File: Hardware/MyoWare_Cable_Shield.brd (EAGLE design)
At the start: 52.3 x 20.8 mm, 16 parts

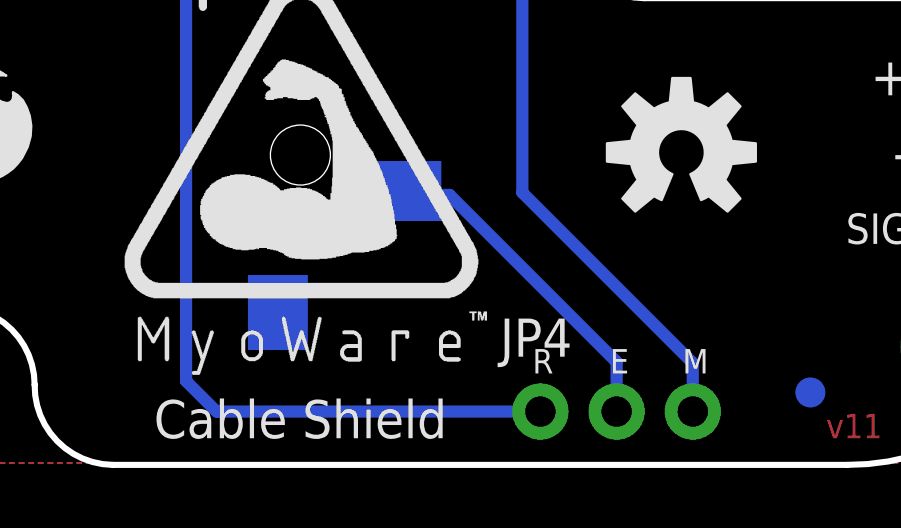
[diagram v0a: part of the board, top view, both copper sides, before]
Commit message: Minor Adjustment
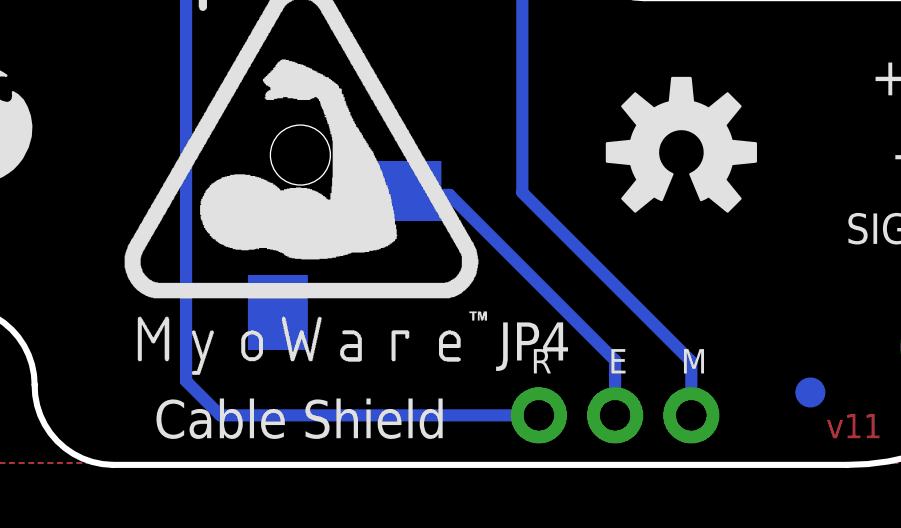
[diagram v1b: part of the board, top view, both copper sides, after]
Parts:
- moved JP4 0.14 mm to (34.1, 1.65)
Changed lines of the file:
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@@
 <?xml version="1.0" encoding="utf-8"?>
 <!DOCTYPE eagle SYSTEM "eagle.dtd">
-<eagle version="7.2.0">
+<eagle version="7.7.0">
 <drawing>
 <settings>
@@
 <wire x1="19.90725" y1="0" x2="44.3865" y2="0" width="0.2032" layer="20"/>
 <wire x1="32.41675" y1="20.828" x2="7.9375" y2="20.828" width="0.2032" layer="20"/>
-<text x="39.3319" y="3.048" size="0.8128" layer="21" font="vector" ratio="20" align="bottom-center">M</text>
-<text x="34.24555" y="3.048" size="0.8128" layer="21" font="vector" ratio="20" align="bottom-center">R</text>
-<text x="36.79825" y="3.048" size="0.8128" layer="21" font="vector" ratio="20" align="bottom-center">E</text>
+<text x="39.2811" y="3.048" size="0.8128" layer="21" font="vector" ratio="20" align="bottom-center">M</text>
+<text x="34.19475" y="3.048" size="0.8128" layer="21" font="vector" ratio="20" align="bottom-center">R</text>
+<text x="36.74745" y="3.048" size="0.8128" layer="21" font="vector" ratio="20" align="bottom-center">E</text>
 <text x="6.4262" y="12.954" size="1.016" layer="21" font="vector" ratio="17" align="center-left">RAW</text>
 <text x="6.4262" y="10.414" size="1.016" layer="21" font="vector" ratio="17" align="center-left">SHLD</text>
@@
 <text x="6.2738" y="10.414" size="1.016" layer="22" font="vector" ratio="17" rot="MR0" align="center-right">SHLD</text>
 <text x="6.2738" y="7.874" size="1.016" layer="22" font="vector" ratio="17" rot="MR0" align="center-right">GND</text>
-<text x="39.17315" y="3.048" size="0.8128" layer="22" font="vector" ratio="20" rot="MR0" align="bottom-center">M</text>
-<text x="34.09315" y="3.048" size="0.8128" layer="22" font="vector" ratio="20" rot="MR0" align="bottom-center">R</text>
-<text x="36.63315" y="3.048" size="0.8128" layer="22" font="vector" ratio="20" rot="MR0" align="bottom-center">E</text>
+<text x="39.12235" y="3.048" size="0.8128" layer="22" font="vector" ratio="20" rot="MR0" align="bottom-center">M</text>
+<text x="34.04235" y="3.048" size="0.8128" layer="22" font="vector" ratio="20" rot="MR0" align="bottom-center">R</text>
+<text x="36.58235" y="3.048" size="0.8128" layer="22" font="vector" ratio="20" rot="MR0" align="bottom-center">E</text>
 <wire x1="50.673" y1="15.5575" x2="52.324" y2="14.0335" width="0.2032" layer="20" curve="-90"/>
 <dimension x1="-6.25475" y1="-10.414" x2="-18.2245" y2="10.414" x3="-34.29" y3="0" textsize="1.778" textratio="15" layer="47" dtype="vertical" unit="inch"/>
@@
 <element name="LOGO" library="advancer-technologies" package="MYOWARE_LOGO" value="" x="26.162" y="9.525"/>
 <element name="SPIRAL" library="advancer-technologies" package="SPIRAL_LOGO_60%" value="" x="22.9489" y="17.7927"/>
-<element name="JP4" library="SparkFun-Connectors" package="1X03_NO_SILK" value="Power" x="34.163" y="1.778"/>
+<element name="JP4" library="SparkFun-Connectors" package="1X03_NO_SILK" value="Power" x="34.1122" y="1.651"/>
 <element name="JP5" library="SparkFun-Connectors" package="1X03_NO_SILK" value="Power" x="50.7365" y="12.954" rot="R270"/>
 <element name="JP2" library="SparkFun-Connectors" package="1X03_NO_SILK" value="Power" x="1.5875" y="12.954" rot="R270"/>
@@
 <contactref element="JP4" pad="3"/>
 <wire x1="33.55975" y1="16.98625" x2="33.55975" y2="9.077959375" width="0.4064" layer="16"/>
-<wire x1="33.55975" y1="9.077959375" x2="39.243" y2="3.394709375" width="0.4064" layer="16"/>
+<wire x1="33.55975" y1="9.077959375" x2="39.1922" y2="3.445509375" width="0.4064" layer="16"/>
 <contactref element="JP3" pad="SLEEVE"/>
 <wire x1="29.612" y1="18.428" x2="32.118" y2="18.428" width="0.4064" layer="16"/>
 <wire x1="32.118" y1="18.428" x2="33.55975" y2="16.98625" width="0.4064" layer="16"/>
-<wire x1="39.243" y1="1.778" x2="39.243" y2="3.394709375" width="0.4064" layer="16"/>
+<wire x1="39.1922" y1="1.651" x2="39.1922" y2="3.445509375" width="0.4064" layer="16"/>
 </signal>
 <signal name="END">
 <contactref element="JP4" pad="2"/>
-<wire x1="36.703" y1="3.429" x2="31.133034375" y2="8.999" width="0.4064" layer="16"/>
+<wire x1="36.6522" y1="3.4798" x2="31.133034375" y2="8.999" width="0.4064" layer="16"/>
 <contactref element="JP3" pad="TIP"/>
 <wire x1="31.133034375" y1="8.999" x2="29.61513125" y2="8.999" width="0.4064" layer="16"/>
 <wire x1="29.61513125" y1="8.999" x2="29.612" y2="9.128" width="0.4064" layer="16"/>
-<wire x1="36.703" y1="1.778" x2="36.703" y2="3.429" width="0.4064" layer="16"/>
+<wire x1="36.6522" y1="1.651" x2="36.6522" y2="3.4798" width="0.4064" layer="16"/>
 </signal>
 <signal name="VREF">
 <contactref element="JP4" pad="1"/>
-<wire x1="34.163" y1="1.778" x2="23.368" y2="1.778" width="0.4064" layer="16"/>
-<wire x1="23.368" y1="1.778" x2="22.352" y2="2.794" width="0.4064" layer="16"/>
+<wire x1="34.1122" y1="1.651" x2="23.495" y2="1.651" width="0.4064" layer="16"/>
+<wire x1="23.495" y1="1.651" x2="22.352" y2="2.794" width="0.4064" layer="16"/>
 <wire x1="22.352" y1="2.794" x2="22.352" y2="16.389" width="0.4064" layer="16"/>
 <contactref element="JP3" pad="RING"/>

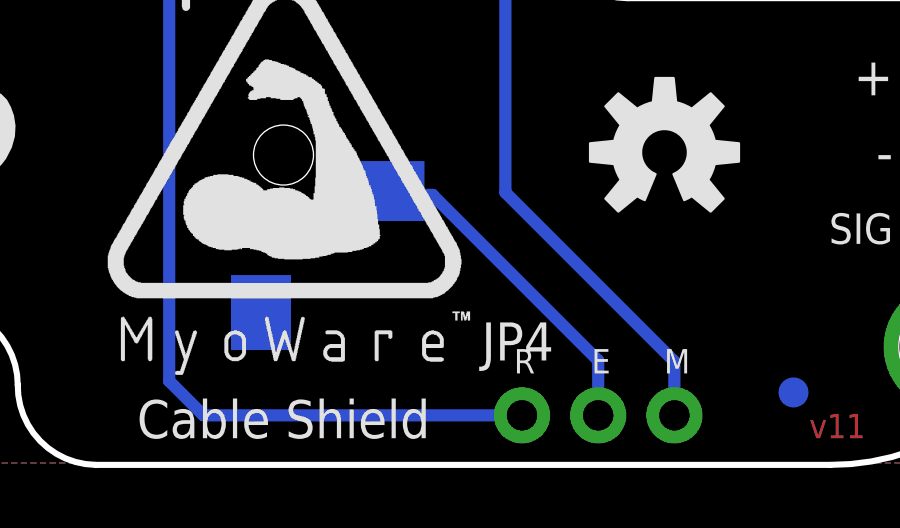
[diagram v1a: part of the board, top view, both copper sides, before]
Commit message: Final Adjust before Protos
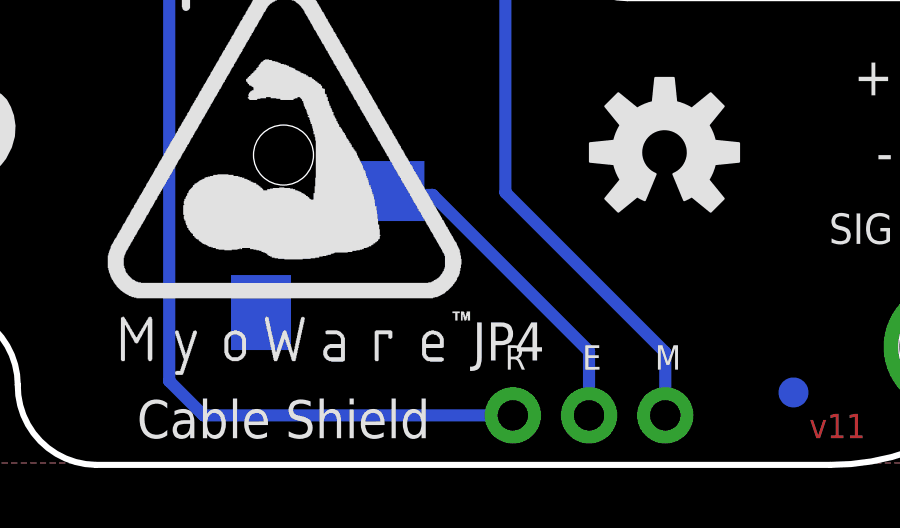
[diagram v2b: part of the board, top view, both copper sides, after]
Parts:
- moved JP4 0.30 mm to (33.8, 1.65)
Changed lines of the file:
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@@
 <?xml version="1.0" encoding="utf-8"?>
 <!DOCTYPE eagle SYSTEM "eagle.dtd">
-<eagle version="7.7.0">
+<eagle version="7.2.0">
 <drawing>
 <settings>
@@
 <wire x1="19.90725" y1="0" x2="44.3865" y2="0" width="0.2032" layer="20"/>
 <wire x1="32.41675" y1="20.828" x2="7.9375" y2="20.828" width="0.2032" layer="20"/>
-<text x="39.2811" y="3.048" size="0.8128" layer="21" font="vector" ratio="20" align="bottom-center">M</text>
-<text x="34.19475" y="3.048" size="0.8128" layer="21" font="vector" ratio="20" align="bottom-center">R</text>
-<text x="36.74745" y="3.048" size="0.8128" layer="21" font="vector" ratio="20" align="bottom-center">E</text>
+<text x="38.9763" y="3.175" size="0.8128" layer="21" font="vector" ratio="20" align="bottom-center">M</text>
+<text x="33.88995" y="3.175" size="0.8128" layer="21" font="vector" ratio="20" align="bottom-center">R</text>
+<text x="36.44265" y="3.175" size="0.8128" layer="21" font="vector" ratio="20" align="bottom-center">E</text>
 <text x="6.4262" y="12.954" size="1.016" layer="21" font="vector" ratio="17" align="center-left">RAW</text>
 <text x="6.4262" y="10.414" size="1.016" layer="21" font="vector" ratio="17" align="center-left">SHLD</text>
@@
 <text x="6.2738" y="10.414" size="1.016" layer="22" font="vector" ratio="17" rot="MR0" align="center-right">SHLD</text>
 <text x="6.2738" y="7.874" size="1.016" layer="22" font="vector" ratio="17" rot="MR0" align="center-right">GND</text>
-<text x="39.12235" y="3.048" size="0.8128" layer="22" font="vector" ratio="20" rot="MR0" align="bottom-center">M</text>
-<text x="34.04235" y="3.048" size="0.8128" layer="22" font="vector" ratio="20" rot="MR0" align="bottom-center">R</text>
-<text x="36.58235" y="3.048" size="0.8128" layer="22" font="vector" ratio="20" rot="MR0" align="bottom-center">E</text>
+<text x="38.81755" y="3.175" size="0.8128" layer="22" font="vector" ratio="20" rot="MR0" align="bottom-center">M</text>
+<text x="33.73755" y="3.175" size="0.8128" layer="22" font="vector" ratio="20" rot="MR0" align="bottom-center">R</text>
+<text x="36.27755" y="3.175" size="0.8128" layer="22" font="vector" ratio="20" rot="MR0" align="bottom-center">E</text>
 <wire x1="50.673" y1="15.5575" x2="52.324" y2="14.0335" width="0.2032" layer="20" curve="-90"/>
 <dimension x1="-6.25475" y1="-10.414" x2="-18.2245" y2="10.414" x3="-34.29" y3="0" textsize="1.778" textratio="15" layer="47" dtype="vertical" unit="inch"/>
@@
 <element name="LOGO" library="advancer-technologies" package="MYOWARE_LOGO" value="" x="26.162" y="9.525"/>
 <element name="SPIRAL" library="advancer-technologies" package="SPIRAL_LOGO_60%" value="" x="22.9489" y="17.7927"/>
-<element name="JP4" library="SparkFun-Connectors" package="1X03_NO_SILK" value="Power" x="34.1122" y="1.651"/>
+<element name="JP4" library="SparkFun-Connectors" package="1X03_NO_SILK" value="Power" x="33.8074" y="1.651"/>
 <element name="JP5" library="SparkFun-Connectors" package="1X03_NO_SILK" value="Power" x="50.7365" y="12.954" rot="R270"/>
 <element name="JP2" library="SparkFun-Connectors" package="1X03_NO_SILK" value="Power" x="1.5875" y="12.954" rot="R270"/>
@@
 <contactref element="JP4" pad="3"/>
 <wire x1="33.55975" y1="16.98625" x2="33.55975" y2="9.077959375" width="0.4064" layer="16"/>
-<wire x1="33.55975" y1="9.077959375" x2="39.1922" y2="3.445509375" width="0.4064" layer="16"/>
+<wire x1="33.55975" y1="9.077959375" x2="38.8874" y2="3.750309375" width="0.4064" layer="16"/>
 <contactref element="JP3" pad="SLEEVE"/>
 <wire x1="29.612" y1="18.428" x2="32.118" y2="18.428" width="0.4064" layer="16"/>
 <wire x1="32.118" y1="18.428" x2="33.55975" y2="16.98625" width="0.4064" layer="16"/>
-<wire x1="39.1922" y1="1.651" x2="39.1922" y2="3.445509375" width="0.4064" layer="16"/>
+<wire x1="38.8874" y1="1.651" x2="38.8874" y2="3.750309375" width="0.4064" layer="16"/>
 </signal>
 <signal name="END">
 <contactref element="JP4" pad="2"/>
-<wire x1="36.6522" y1="3.4798" x2="31.133034375" y2="8.999" width="0.4064" layer="16"/>
+<wire x1="36.3474" y1="3.7846" x2="31.133034375" y2="8.999" width="0.4064" layer="16"/>
 <contactref element="JP3" pad="TIP"/>
 <wire x1="31.133034375" y1="8.999" x2="29.61513125" y2="8.999" width="0.4064" layer="16"/>
 <wire x1="29.61513125" y1="8.999" x2="29.612" y2="9.128" width="0.4064" layer="16"/>
-<wire x1="36.6522" y1="1.651" x2="36.6522" y2="3.4798" width="0.4064" layer="16"/>
+<wire x1="36.3474" y1="1.651" x2="36.3474" y2="3.7846" width="0.4064" layer="16"/>
 </signal>
 <signal name="VREF">
 <contactref element="JP4" pad="1"/>
-<wire x1="34.1122" y1="1.651" x2="23.495" y2="1.651" width="0.4064" layer="16"/>
+<wire x1="33.8074" y1="1.651" x2="23.495" y2="1.651" width="0.4064" layer="16"/>
 <wire x1="23.495" y1="1.651" x2="22.352" y2="2.794" width="0.4064" layer="16"/>
 <wire x1="22.352" y1="2.794" x2="22.352" y2="16.389" width="0.4064" layer="16"/>
